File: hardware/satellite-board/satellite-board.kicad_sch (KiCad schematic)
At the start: 27 parts, among them J1 MTJ-88ARX1-FSM-LG, J2 B2B-PH-K-S, Q1 2N7002, U1 LORA1262-915TCXO, U2 XC6220B331MR, U3 ESP32-C6-DEVKITC-1-N8, U4 MAX3485

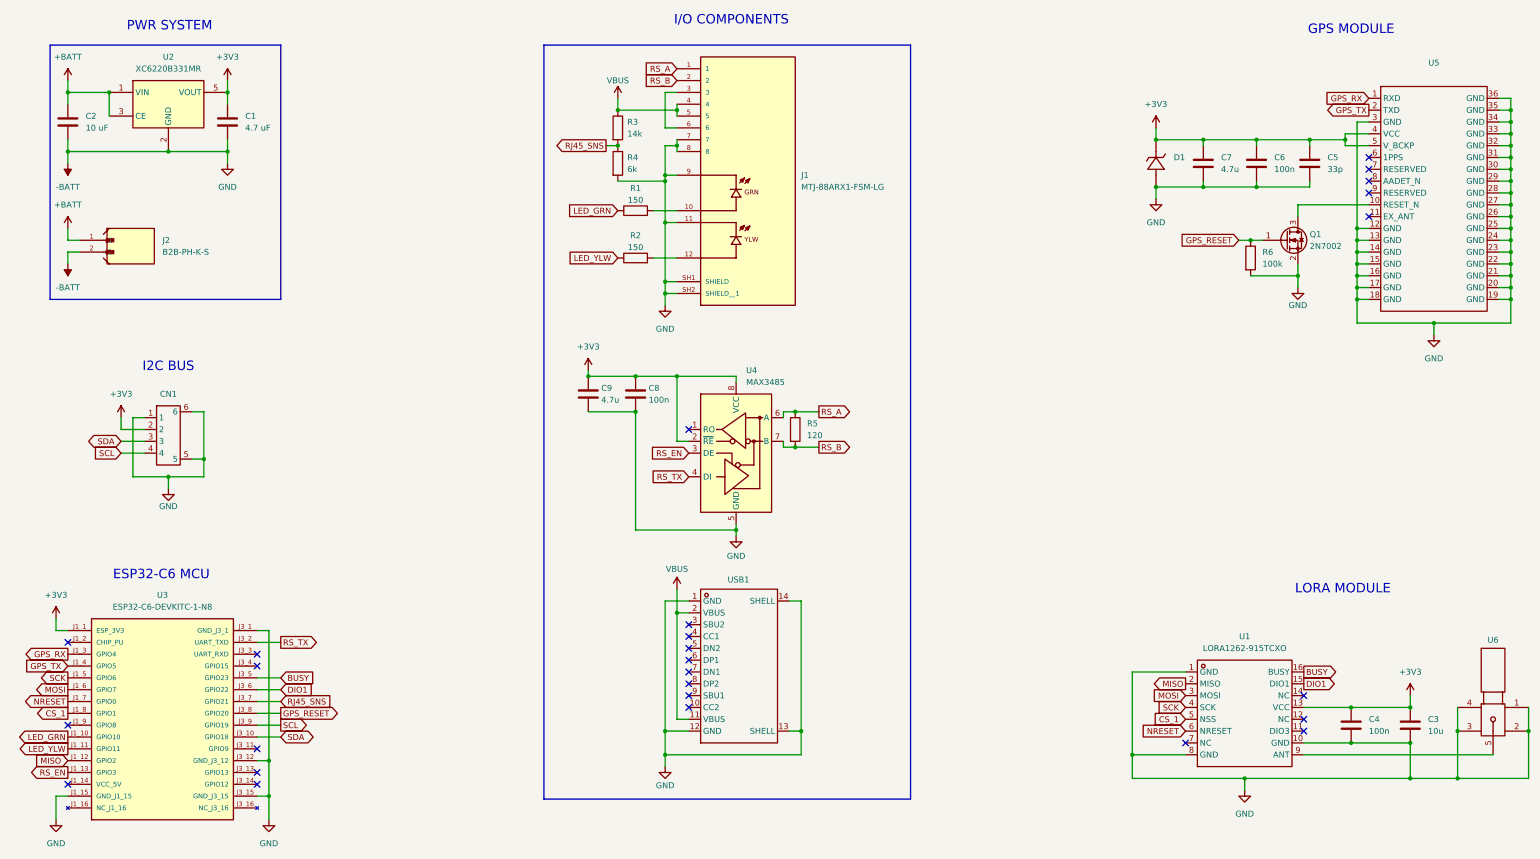
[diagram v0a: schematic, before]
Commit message: Satelite & Central Schematic Finished
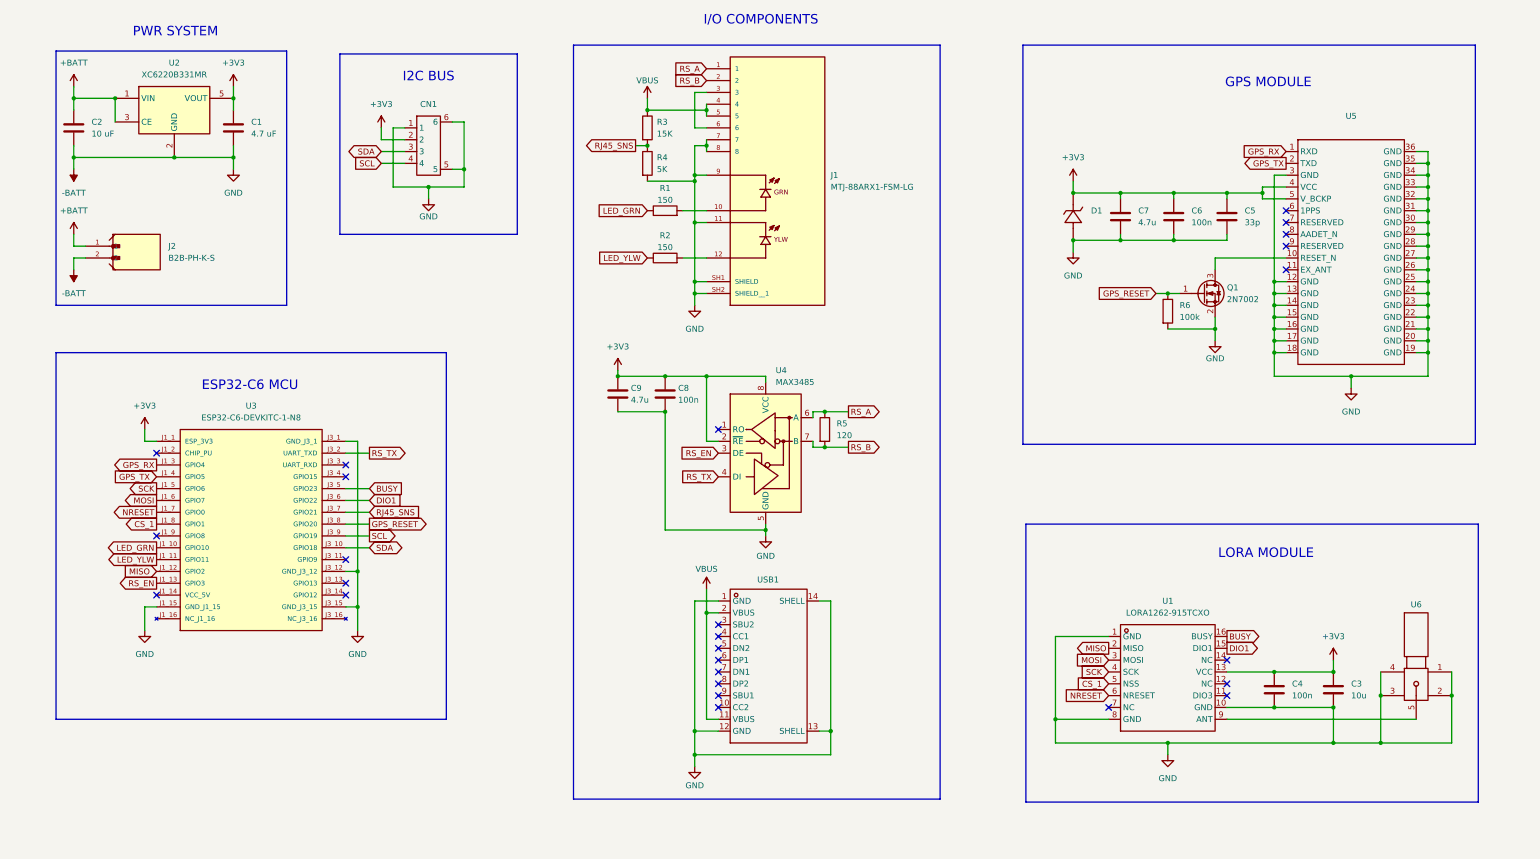
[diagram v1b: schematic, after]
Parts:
- R3: value 14k -> 15K
- R4: value 6k -> 5K
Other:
- moved on the sheet: C1, C2, C3, C4, C5, C6, C7, C8, C9, CN1, D1, J1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
